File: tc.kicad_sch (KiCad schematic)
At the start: 9 parts

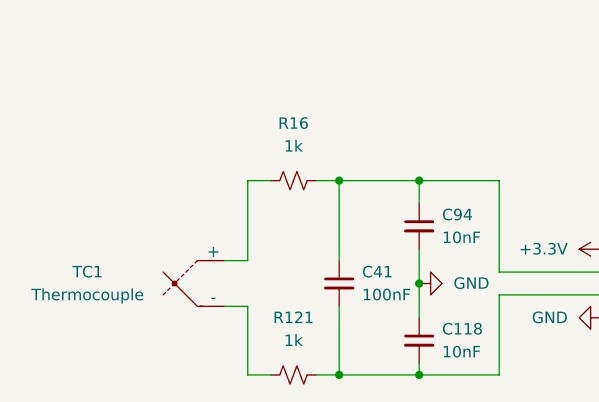
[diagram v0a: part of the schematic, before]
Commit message: version in PCBway 12/12/2025
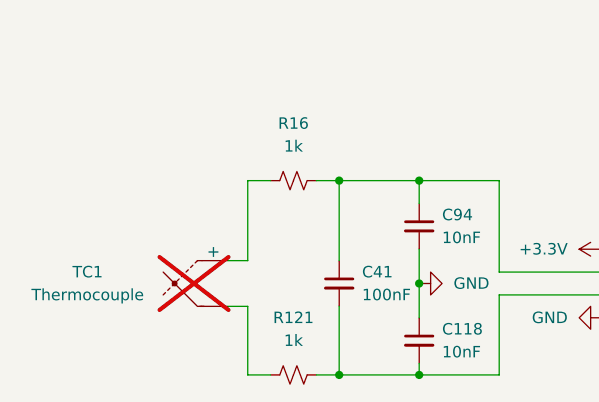
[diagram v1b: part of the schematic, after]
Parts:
- C41: Part # Generic CAP CER 10NF 6.3V X7R 0402 -> Generic CAP CER 0.1UF 6.3V X7R 0402
- R121, R16: Part # (none) -> Generic RES SMD 1K OHM 1% 1/16W 0402
- TC1: now not fitted
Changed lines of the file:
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@@
 		(in_bom yes)
 		(on_board yes)
-		(dnp no)
+		(dnp yes)
 		(property "Reference" "TC1"
 			(at 85.09 100.33 0)
@@
 			)
 		)
+		(property "Part #" "Generic RES SMD 1K OHM 1% 1/16W 0402"
+			(at 107.95 111.76 90)
+			(effects
+				(font
+					(size 1.27 1.27)
+				)
+				(hide yes)
+			)
+		)
 		(pin "2"
 		)
@@
 			)
 		)
-		(property "Part #" "Generic CAP CER 10NF 6.3V X7R 0402"
+		(property "Part #" "Generic CAP CER 0.1UF 6.3V X7R 0402"
 			(at 113.03 101.6 0)
 			(effects
@@
 			(effects
 				(font
+					(size 1.27 1.27)
+				)
+				(hide yes)
+			)
+		)
+		(property "Part #" "Generic RES SMD 1K OHM 1% 1/16W 0402"
+			(at 107.95 90.17 90)
+			(effects
+				(font
